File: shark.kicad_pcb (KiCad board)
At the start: 2 copper layers, 226.2 x 78.2 mm, 236 parts, among them J101 USB_B_Mini, Q1 AO4406AL, SW1 MXSwitch, SW10 MXSwitch, SW11 MXSwitch, SW12 MXSwitch, SW13 MXSwitch, SW14 MXSwitch, SW15 MXSwitch, SW16 MXSwitch, SW17 MXSwitch, SW18 MXSwitch, SW19 MXSwitch, SW2 MXSwitch, SW20 MXSwitch, SW21 MXSwitch, SW22 MXSwitch, SW23 MXSwitch, SW24 MXSwitch, SW25 MXSwitch, SW26 MXSwitch, SW27 MXSwitch, SW28 MXSwitch, SW29 MXSwitch, SW3 MXSwitch, SW30 MXSwitch, SW31 MXSwitch, SW32 MXSwitch, SW33 MXSwitch, SW34 MXSwitch, SW35 MXSwitch, SW36 MXSwitch, SW37 MXSwitch, SW38 MXSwitch, SW39 MXSwitch, SW4 MXSwitch, SW40 MXSwitch, SW41 MXSwitch, SW42 MXSwitch, SW43 MXSwitch, SW44 MXSwitch, SW45 MXSwitch, SW46 MXSwitch, SW47 MXSwitch, SW48 MXSwitch, SW49 MXSwitch, SW5 MXSwitch, SW50 MXSwitch, SW51 MXSwitch, SW6 MXSwitch, SW7 MXSwitch, SW8 MXSwitch, SW9 MXSwitch, U1 ATmega32U4-AU, Y1 Crystal

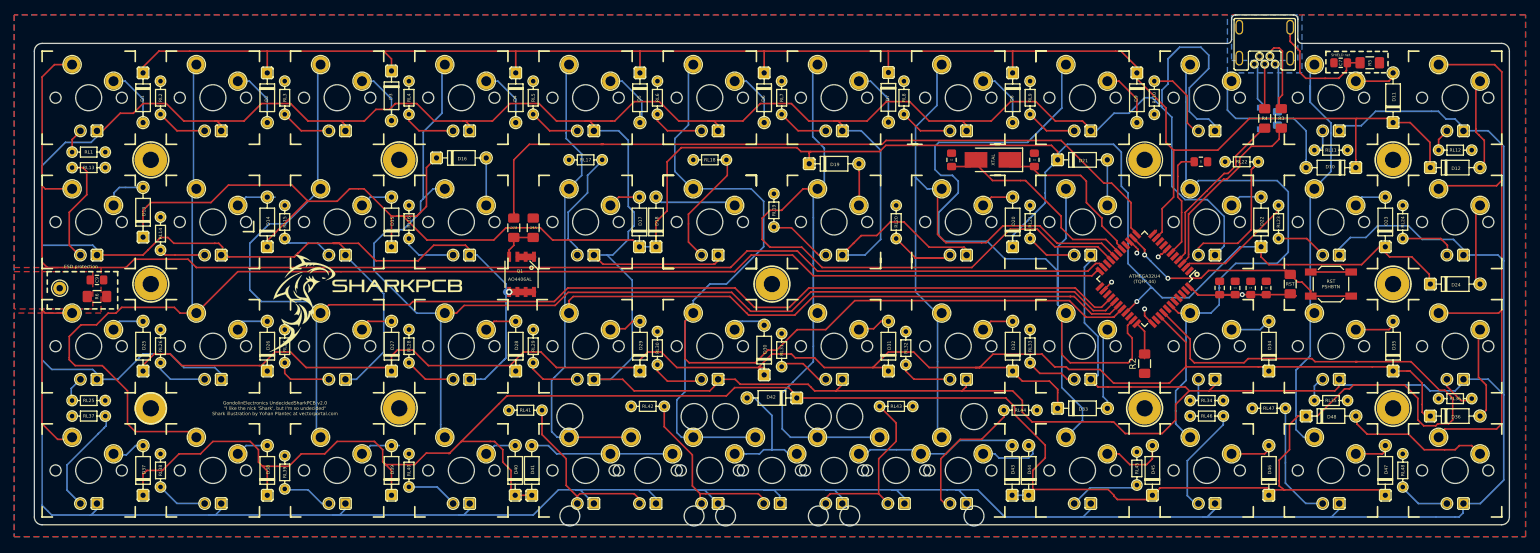
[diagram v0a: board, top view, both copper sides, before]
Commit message: Began porting to STM32
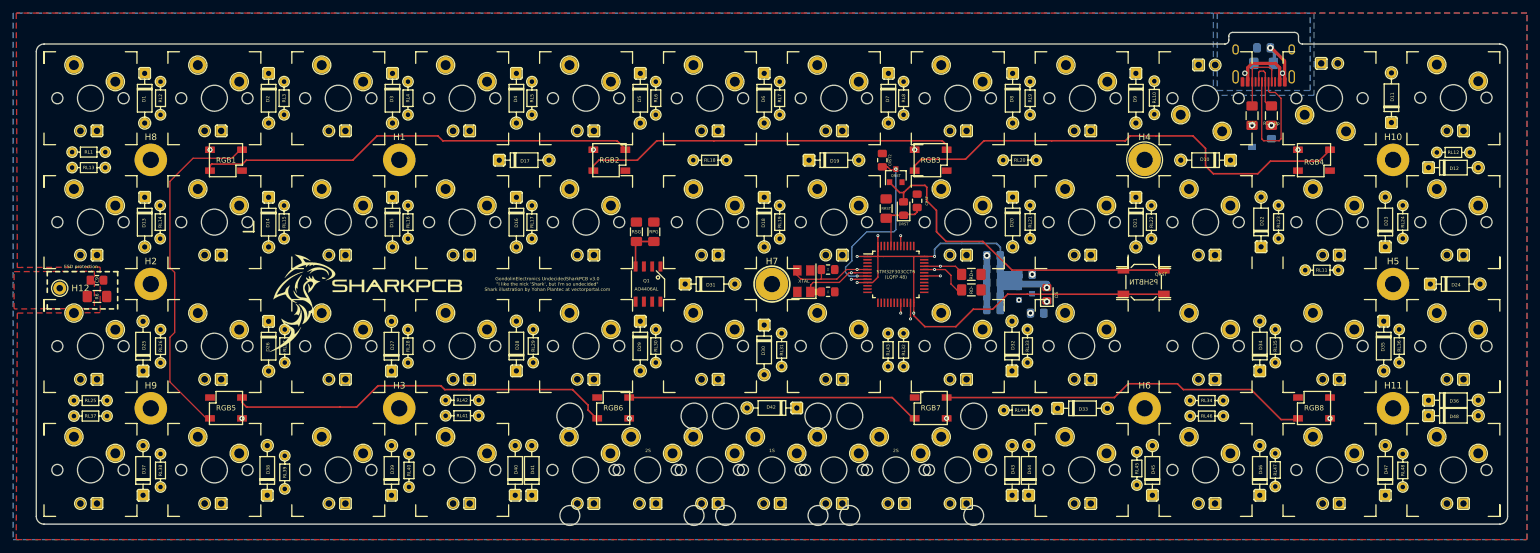
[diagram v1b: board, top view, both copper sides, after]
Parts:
- removed C3, C4, C5: 0.1u, Capacitor_SMD:C_0805_2012Metric_Pad1.15x1.40mm_HandSolder
- removed C6: 4.7u, Capacitor_SMD:C_0805_2012Metric_Pad1.15x1.40mm_HandSolder
- removed C8: 1u, Capacitor_SMD:C_0805_2012Metric_Pad1.15x1.40mm_HandSolder
- removed J101: USB_B_Mini, Keyboard_switches:miniB_connector
- removed PSH1: SW_Push, Button_Switch_SMD:SW_SPST_SKQG_WithStem
- removed R1, R2, RPGate101: 10k, Resistor_SMD:R_1206_3216Metric_Pad1.42x1.75mm_HandSolder
- removed R3, R4: 22, Resistor_SMD:R_1206_3216Metric_Pad1.42x1.75mm_HandSolder
- removed RSGate101: 1k, Resistor_SMD:R_1206_3216Metric_Pad1.42x1.75mm_HandSolder
- added CRST1: 4.7n, Capacitor_SMD:C_0805_2012Metric_Pad1.15x1.40mm_HandSolder, F.Cu at (170.7, 90.0)
- added CSRT2: 4.7n, Capacitor_SMD:C_0805_2012Metric_Pad1.15x1.40mm_HandSolder, F.Cu at (165.4, 83.7)
- added CSin1: 100n, Capacitor_SMD:C_0805_2012Metric_Pad1.15x1.40mm_HandSolder, B.Cu at (189.1, 107.2)
- added CSout1: 100n, Capacitor_SMD:C_0805_2012Metric_Pad1.15x1.40mm_HandSolder, B.Cu at (187.4, 101.3)
- added CVBus1: 100n, Capacitor_SMD:C_0805_2012Metric_Pad1.15x1.40mm_HandSolder, B.Cu at (182.4, 102.5)
- added CVBus2: 100n, Capacitor_SMD:C_0805_2012Metric_Pad1.15x1.40mm_HandSolder, B.Cu at (182.4, 104.6)
- added CVBus3: 100n, Capacitor_SMD:C_0805_2012Metric_Pad1.15x1.40mm_HandSolder, B.Cu at (182.4, 100.4)
- added CVBus4: 1u, Capacitor_SMD:C_0805_2012Metric_Pad1.15x1.40mm_HandSolder, B.Cu at (182.4, 106.7)
- added CVBus5: 4.7u, Capacitor_SMD:C_0805_2012Metric_Pad1.15x1.40mm_HandSolder, B.Cu at (182.4, 98.4)
- added DF1: RB060M-60TR, Diode_SMD:D_SOD-123, B.Cu at (222.1, 80.0)
- added DRST1: 1N4148, Diode_SMD:D_0805_2012Metric_Pad1.15x1.40mm_HandSolder, F.Cu at (168.7, 91.2)
- added J1: USB_C_Receptacle, USBconnector:TYPE-C-31-M-13, F.Cu at (223.9, 72.5)
- added QRST1: BC847, Package_TO_SOT_SMD:SOT-23, F.Cu at (167.5, 86.1)
- added RCC1: 5.1k, Resistor_SMD:R_1206_3216Metric_Pad1.42x1.75mm_HandSolder, F.Cu at (222.1, 76.9)
- added RD+1: 22R, Resistor_SMD:R_1206_3216Metric_Pad1.42x1.75mm_HandSolder, F.Cu at (179.0, 101.3)
- added RD+Up1: 1.5k, Resistor_SMD:R_1206_3216Metric_Pad1.42x1.75mm_HandSolder, F.Cu at (225.1, 76.9)
- added RD-1: 22R, Resistor_SMD:R_1206_3216Metric_Pad1.42x1.75mm_HandSolder, F.Cu at (179.0, 103.6)
- added RGB1: WS2812B, Keyboard_switches:LED_WS2812B, F.Cu at (64.7, 83.7)
- added RGB2: WS2812B, Keyboard_switches:LED_WS2812B, F.Cu at (123.5, 83.7)
- added RGB3: WS2812B, Keyboard_switches:LED_WS2812B, F.Cu at (172.8, 83.7)
- added RGB4: WS2812B, Keyboard_switches:LED_WS2812B, F.Cu at (231.6, 83.7)
- added RGB5: WS2812B, Keyboard_switches:LED_WS2812B, F.Cu at (64.7, 121.7)
- added RGB6: WS2812B, Keyboard_switches:LED_WS2812B, F.Cu at (124.1, 121.7)
- added RGB7: WS2812B, Keyboard_switches:LED_WS2812B, F.Cu at (172.8, 121.7)
- added RGB8: WS2812B, Keyboard_switches:LED_WS2812B, F.Cu at (231.6, 121.7)
- added RPGate1: 10k, Resistor_SMD:R_1206_3216Metric_Pad1.42x1.75mm_HandSolder, F.Cu at (130.4, 94.7)
- added RRST1: 100k, Resistor_SMD:R_1206_3216Metric_Pad1.42x1.75mm_HandSolder, F.Cu at (166.0, 91.2)
- added RSGate1: 1k, Resistor_SMD:R_1206_3216Metric_Pad1.42x1.75mm_HandSolder, F.Cu at (127.7, 94.7)
- added SWRST1: SW_Push, Button_Switch_SMD:SW_SPST_SKQG_WithoutStem, F.Cu at (205.5, 102.4)
- added U2: MCP1700-3302E_SOT23, Package_TO_SOT_SMD:SOT-23, B.Cu at (187.4, 104.2)
- C7, R5: moved to B.Cu
- DS1: value RB060M-60TR -> 1N4148; footprint Diode_SMD:D_SOD-123 -> Diode_SMD:D_0805_2012Metric_Pad1.15x1.40mm_HandSolder; moved to F.Cu
- U1: value ATmega32U4-AU -> STM32F303CCT7; footprint Package_QFP:TQFP-44_10x10mm_P0.8mm -> Package_QFP:LQFP-48_7x7mm_P0.5mm
- Y1: value Crystal -> 8MHz; footprint Crystal:Crystal_SMD_5032-2Pin_5.0x3.2mm_HandSoldering -> Crystal:Crystal_SMD_5032-4Pin_5.0x3.2mm
- moved DS1 42.5 mm to (190.6, 104.3)
- moved U1 38.2 mm to (167.5, 101.3), turned to 0 degrees
- moved C1 37.6 mm to (157.1, 103.9), turned to 0 degrees
- moved Y1 34.5 mm to (153.4, 102.3), turned to 90 degrees
- moved D31 29.0 mm to (139.0, 102.7), turned to 0 degrees
- moved RL42 28.5 mm to (101.0, 120.6)
- moved C2 25.3 mm to (157.1, 100.5), turned to 0 degrees
- moved RL20 21.2 mm to (186.5, 83.7), turned to 180 degrees
- moved D17 20.1 mm to (110.5, 83.7), turned to 0 degrees
- moved Q1 19.5 mm to (129.5, 102.7)
- moved D10 19.3 mm to (215.0, 83.7)
- moved D48 18.8 mm to (253.0, 122.9)
- moved RL11 18.5 mm to (232.8, 100.6), turned to 0 degrees
- moved RL22 16.7 mm to (206.7, 93.2), turned to 270 degrees
- moved D18 16.6 mm to (147.3, 93.2), turned to 270 degrees
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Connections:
- DS1 pad 1: VCC -> 5V
- DS1 pad 2: GND -> 3.3V
- F1 pad 1: VCC -> 5V
- F1 pad 2: Net-(F1-Pad2) -> VBUS
- RL1 pad 1: VCC -> 5V
- RL10 pad 1: VCC -> 5V
- RL11 pad 1: VCC -> 5V
- RL12 pad 1: VCC -> 5V
- RL13 pad 1: VCC -> 5V
- RL14 pad 1: VCC -> 5V
- RL15 pad 1: VCC -> 5V
- RL16 pad 1: VCC -> 5V
- RL17 pad 1: VCC -> 5V
- RL18 pad 1: VCC -> 5V
- RL19 pad 1: VCC -> 5V
- RL2 pad 1: VCC -> 5V
- RL20 pad 1: VCC -> 5V
- RL21 pad 1: VCC -> 5V
- RL22 pad 1: VCC -> 5V
- RL23 pad 1: VCC -> 5V
- RL24 pad 1: VCC -> 5V
- RL25 pad 1: VCC -> 5V
- RL26 pad 1: VCC -> 5V
- RL27 pad 1: VCC -> 5V
- RL28 pad 1: VCC -> 5V
- RL29 pad 1: VCC -> 5V
- RL3 pad 1: VCC -> 5V
- RL30 pad 1: VCC -> 5V
- RL31 pad 1: VCC -> 5V
- RL32 pad 1: VCC -> 5V
- RL33 pad 1: VCC -> 5V
- RL34 pad 1: VCC -> 5V
- RL35 pad 1: VCC -> 5V
- RL36 pad 1: VCC -> 5V
- RL37 pad 1: VCC -> 5V
- RL38 pad 1: VCC -> 5V
- RL39 pad 1: VCC -> 5V
- RL4 pad 1: VCC -> 5V
- RL40 pad 1: VCC -> 5V
- RL41 pad 1: VCC -> 5V
- RL42 pad 1: VCC -> 5V
- RL43 pad 1: VCC -> 5V
- RL44 pad 1: VCC -> 5V
- RL45 pad 1: VCC -> 5V
- RL46 pad 1: VCC -> 5V
- RL47 pad 1: VCC -> 5V
- RL48 pad 1: VCC -> 5V
- RL5 pad 1: VCC -> 5V
- RL6 pad 1: VCC -> 5V
- RL7 pad 1: VCC -> 5V
- RL8 pad 1: VCC -> 5V
- RL9 pad 1: VCC -> 5V
- U1 pad 1: (no net) -> 3.3V
- U1 pad 10: Row1 -> (no net)
- U1 pad 12: LED_PWM -> (no net)
- U1 pad 13: RST -> (no net)
- U1 pad 14: VCC -> (no net)
- U1 pad 15: GND -> (no net)
- U1 pad 16: XTAL2 -> (no net)
- U1 pad 17: XTAL1 -> (no net)
- U1 pad 18: Col8 -> (no net)
- U1 pad 19: Col7 -> (no net)
- U1 pad 2: VCC -> (no net)
- U1 pad 20: (no net) -> RGB_PWM
- U1 pad 21: Col1 -> (no net)
- U1 pad 22: Col2 -> (no net)
- U1 pad 24: VCC -> 3.3V
- U1 pad 26: Col3 -> (no net)
- U1 pad 27: Col4 -> (no net)
- U1 pad 28: Col5 -> (no net)
- U1 pad 29: Col6 -> (no net)
- U1 pad 3: Net-(R3-Pad1) -> (no net)
- U1 pad 30: Row2 -> (no net)
- U1 pad 32: Col9 -> D-
- U1 pad 33: Net-(R2-Pad2) -> D+
- U1 pad 34: VCC -> (no net)
- U1 pad 36: Row3 -> 3.3V
- U1 pad 37: Row4 -> (no net)
- U1 pad 39: Col10 -> (no net)
- U1 pad 4: Net-(R4-Pad1) -> (no net)
- U1 pad 41: (no net) -> LED_PWM
- U1 pad 43: GND -> (no net)
- U1 pad 44: VCC -> BOOT0
- U1 pad 5: GND -> XTAL1
- U1 pad 6: Net-(C8-Pad1) -> XTAL2
- U1 pad 7: VCC -> NRST
- U1 pad 8: (no net) -> GND
- U1 pad 9: (no net) -> 3.3V
- Y1 pad 2: XTAL1 -> GND
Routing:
- net Net-(LED1-PadK): track 1206.4 -> 0.00 mm, vias 1 -> 0
- net Row4: track 357.8 -> 0.00 mm
- net Row2: track 309.9 -> 0.00 mm, vias 1 -> 0
- net Row1: track 263.1 -> 0.00 mm
- net Row3: track 259.4 -> 0.00 mm
- net Col1: track 251.2 -> 0.00 mm
- net Col2: track 241.6 -> 0.00 mm
- net Col3: track 206.9 -> 0.00 mm
- net Col4: track 188.2 -> 0.00 mm
- net Col6: track 171.6 -> 0.00 mm
- net Col5: track 167.2 -> 0.00 mm
- net Col7: track 153.4 -> 0.00 mm
- net Col9: track 142.2 -> 0.00 mm
- net 3.3V: track 0.00 -> 116.6 mm, vias 0 -> 6
- net LED_PWM: track 113.8 -> 1.59 mm, vias 0 -> 1
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- added copper zone on B.Cu, net 5V
- removed copper zone on B.Cu, net VCC
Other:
- board size 226.2 x 78.2 mm -> 225.6 x 75.4 mm
- net class Fine added: clearance 0.2, trace_width 0.13, via_dia 0.508, via_drill 0.2032
- board text added: "1S"
- board text added: "2S"
- board text added: "CRST"
- board text added: "CRST2"
- board text added: "CSI"
- board text added: "CSO"
- board text added: "DRST"
- board text added: "DS"
- board text added: "GondolinElectronics UndecidedSharkPCB v3.0 "I like the nick 'Shark', but I'm so undecided" Shark illustration by Yohan Plantec at vectorportal.com"
- board text added: "LDO"
- board text added: "PSHBTN"
- board text added: "QRST"
- board text added: "RCC"
- board text added: "RD+"
- board text added: "RD+Up"
- board text added: "RD-"
- board text added: "RRST"
- board text added: "STM32F303CCT6 (LQFP 48)"
- board text removed: "ATMEGA32U4 (TQFP 44)"
- board text removed: "GondolinElectronics UndecidedSharkPCB v2.0 "I like the nick 'Shark', but I'm so undecided" Shark illustration by Yohan Plantec at vectorportal.com"
- board text removed: "RST"
- board text removed: "RST PSHBTN"
- board text removed: "SHIELD net"
